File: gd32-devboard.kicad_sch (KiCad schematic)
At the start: 0 parts

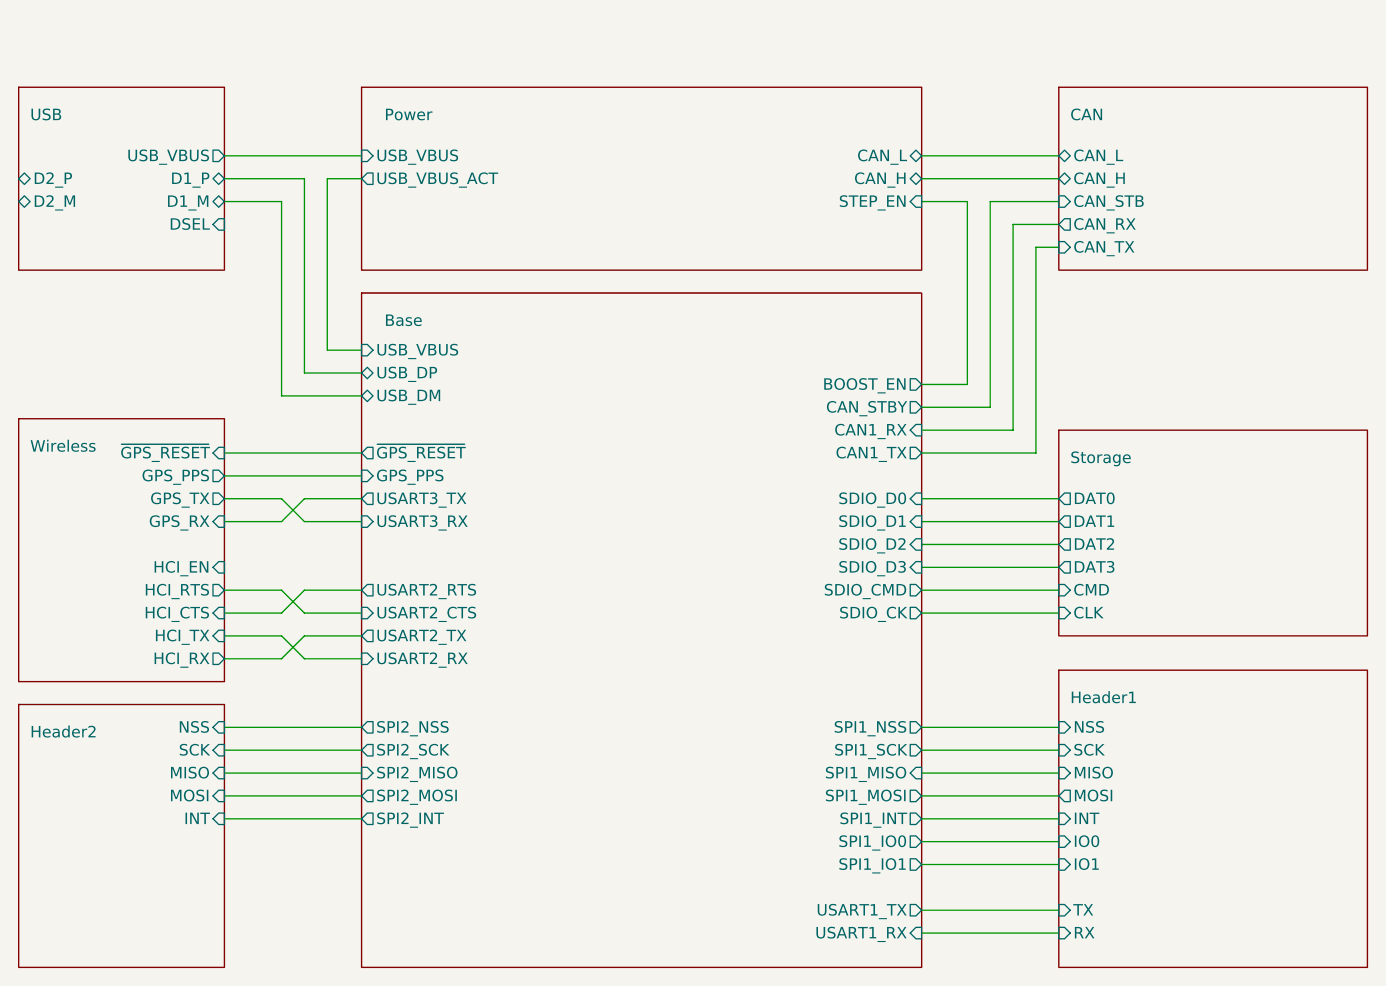
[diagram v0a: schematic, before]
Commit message: production: prepare for fab
Signed-off-by: Connor Rigby <connorr@hey.com>
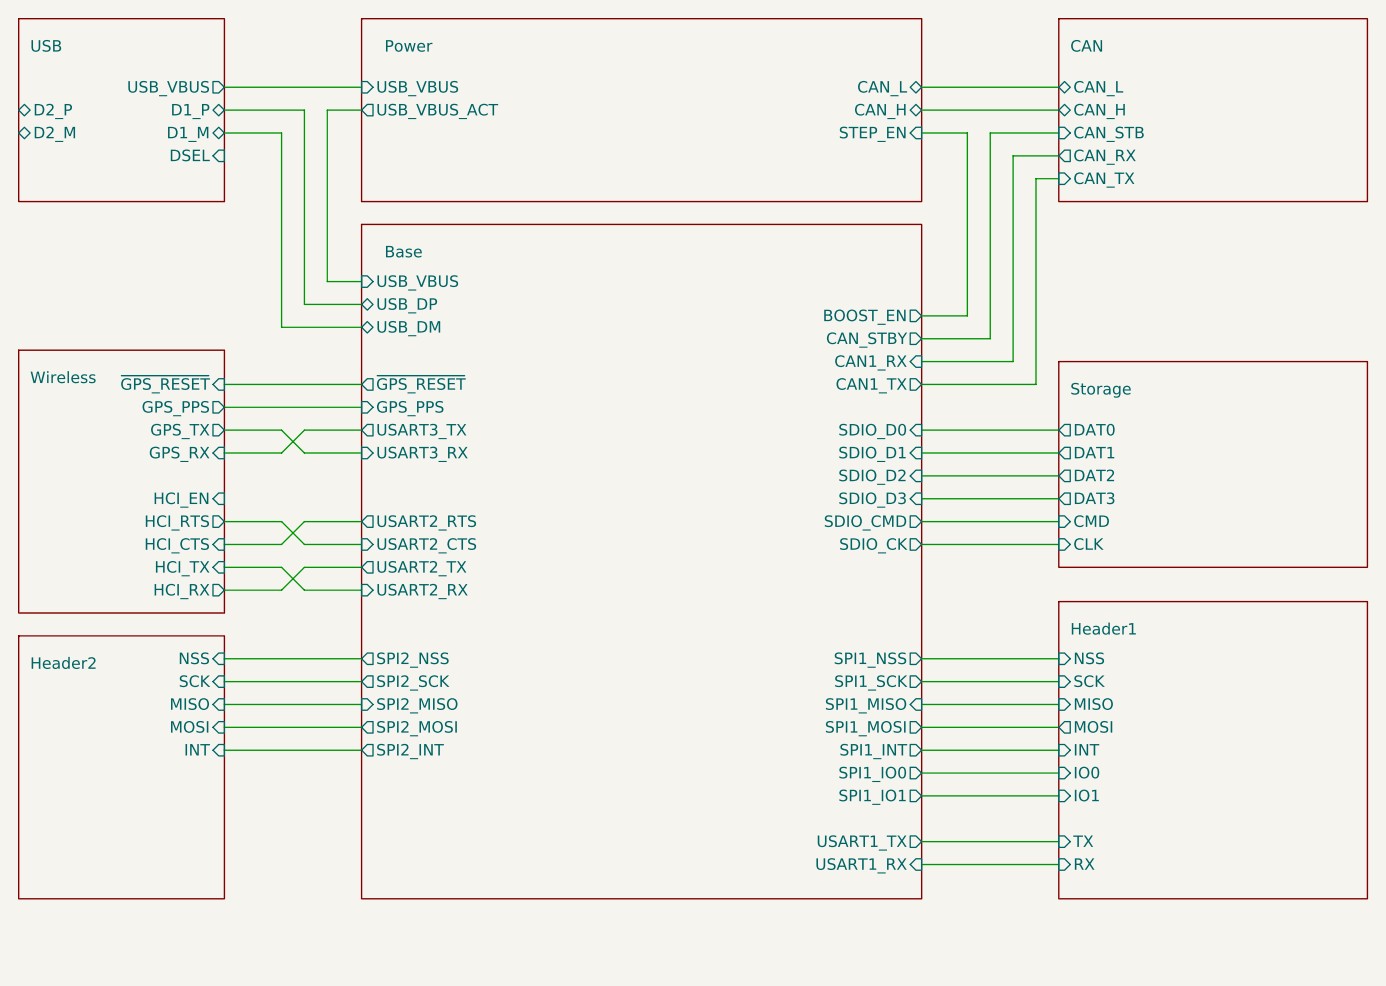
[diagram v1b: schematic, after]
